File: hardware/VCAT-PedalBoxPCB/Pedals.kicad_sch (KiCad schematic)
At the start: 0 parts

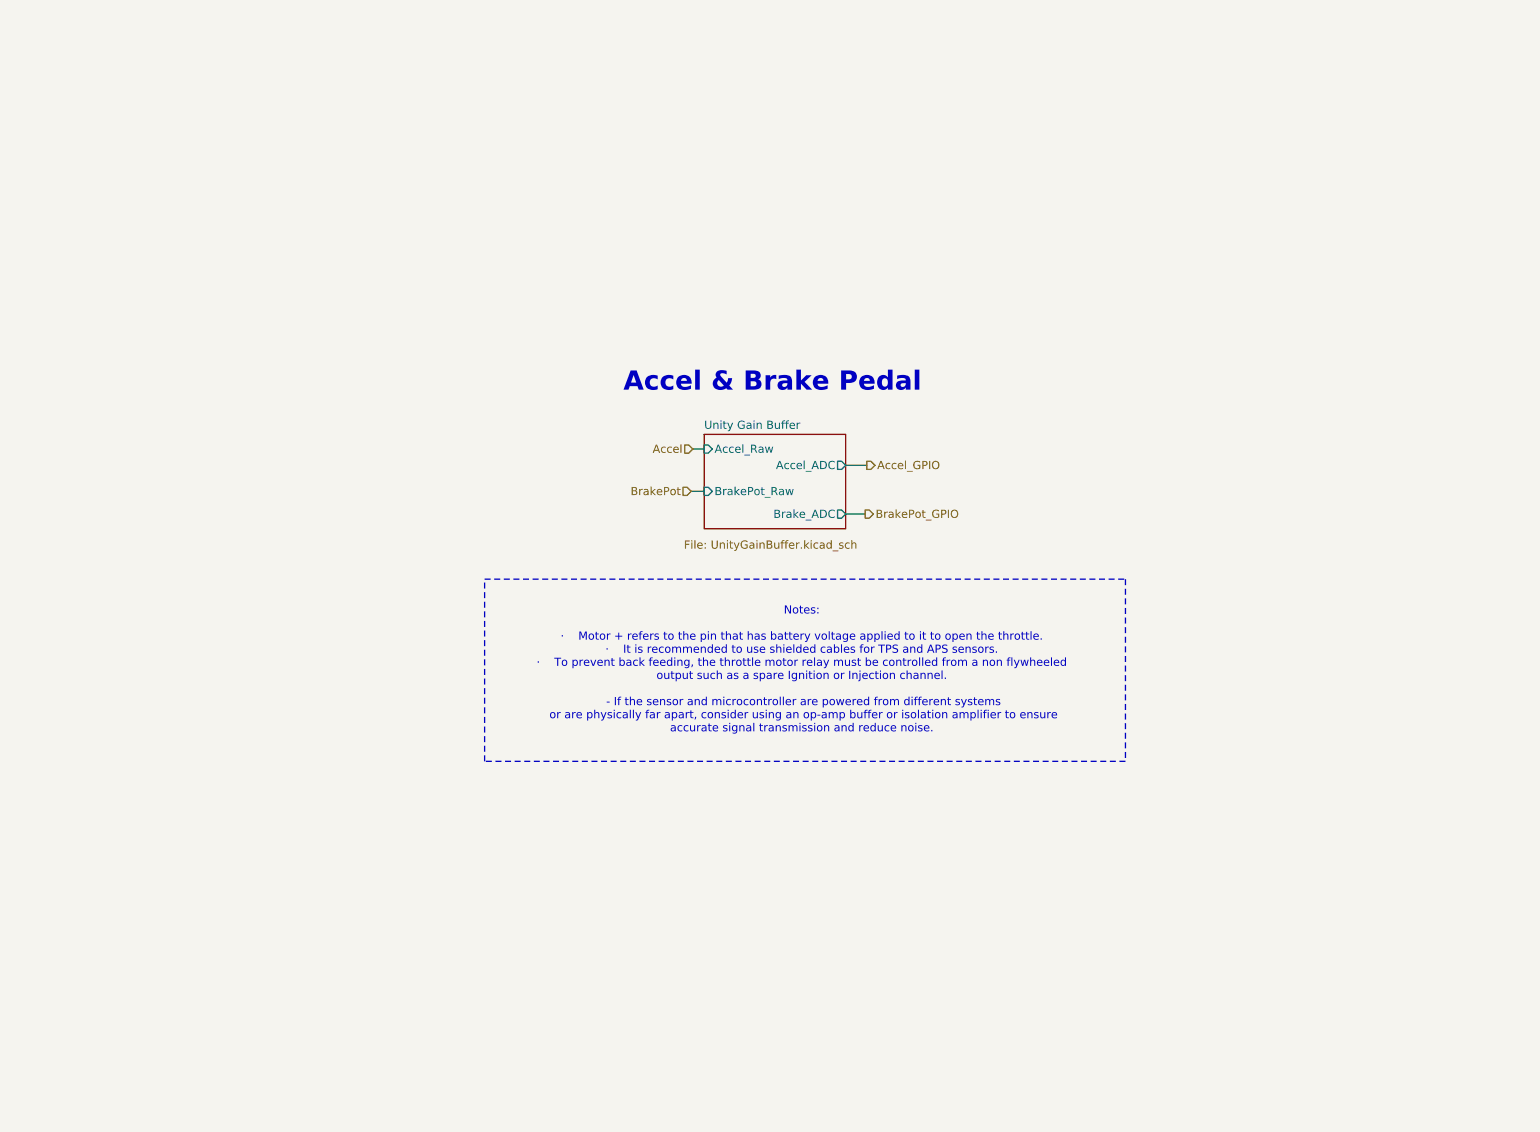
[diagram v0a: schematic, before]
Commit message: Rev B Sch updates
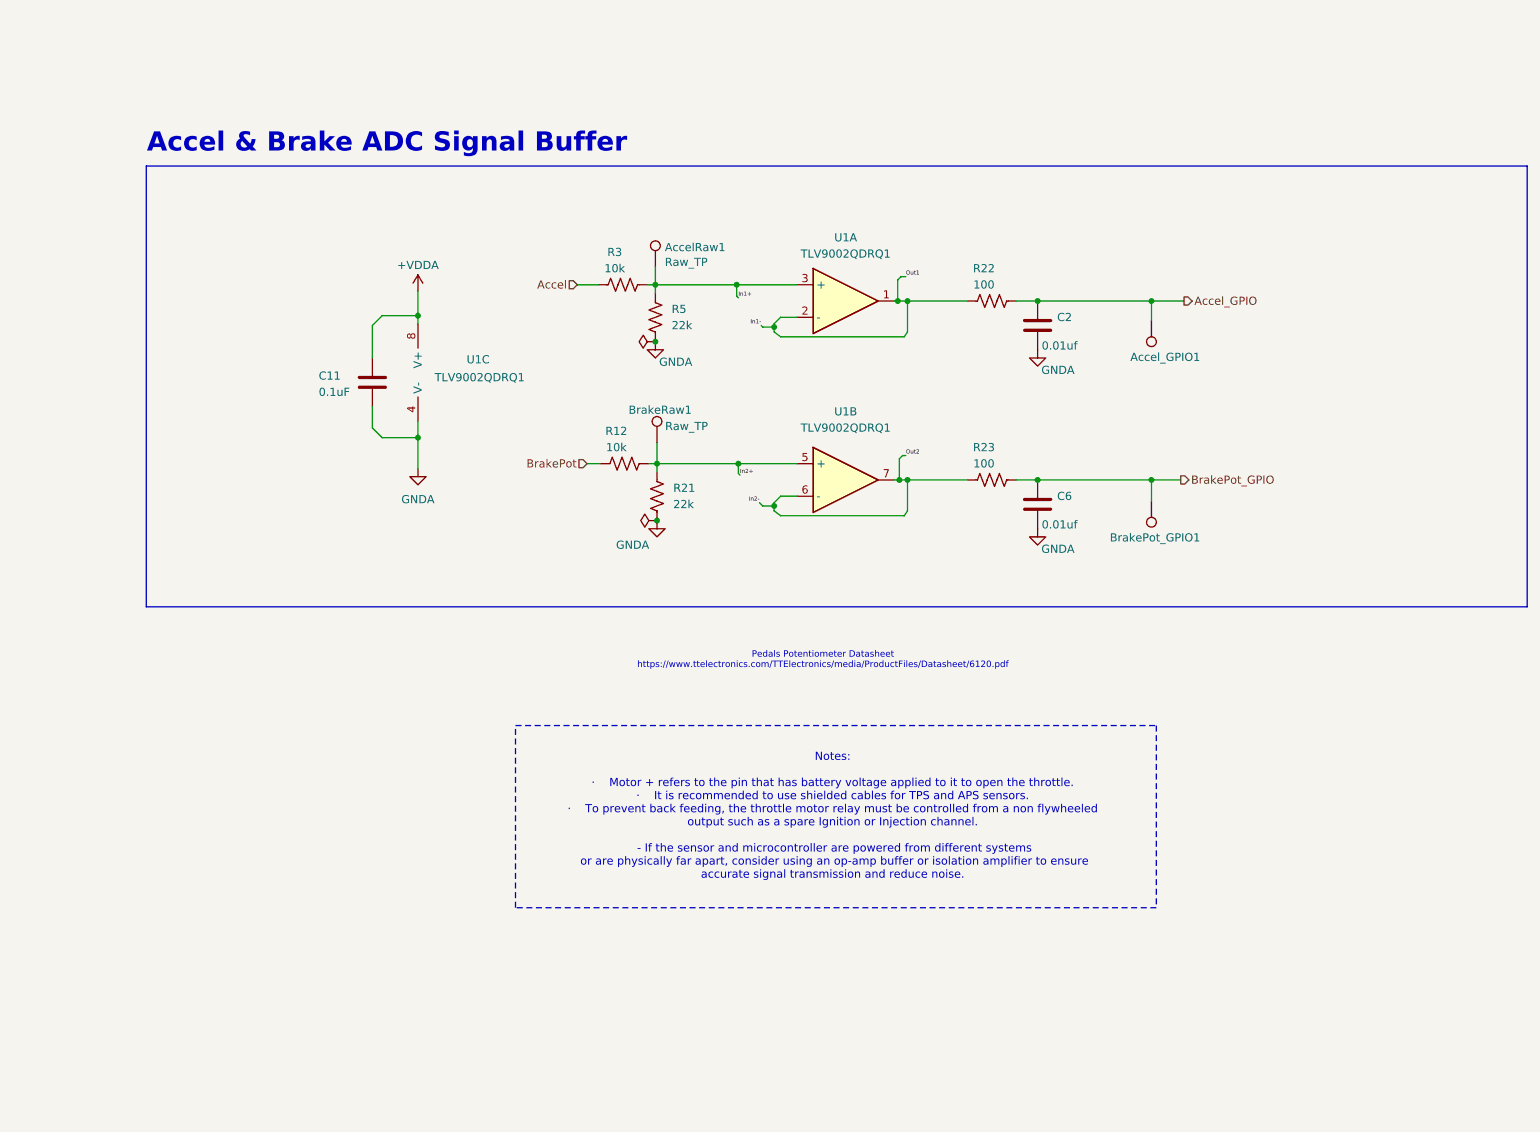
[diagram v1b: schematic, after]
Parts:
- added AccelRaw1, BrakeRaw1: Raw_TP, TestPoint:TestPoint_THTPad_1.5x1.5mm_Drill0.7mm, symbol Connector:TestPoint
- added Accel_GPIO1, BrakePot_GPIO1: Accel, TestPoint:TestPoint_THTPad_1.5x1.5mm_Drill0.7mm, symbol Connector:TestPoint
- added C11: 0.1uF, Capacitor_SMD:C_0603_1608Metric_Pad1.08x0.95mm_HandSolder, symbol Device:C
- added C2, C6: 0.01uf, Capacitor_SMD:C_0603_1608Metric_Pad1.08x0.95mm_HandSolder, symbol Device:C
- added R12, R3: 10k, Resistor_SMD:R_0603_1608Metric_Pad0.98x0.95mm_HandSolder, symbol Device:R_US
- added R21, R5: 22k, Resistor_SMD:R_0603_1608Metric_Pad0.98x0.95mm_HandSolder, symbol Device:R_US
- added R22, R23: 100, Resistor_SMD:R_0603_1608Metric_Pad0.98x0.95mm_HandSolder, symbol Device:R_US
- added U1: TLV9002QDRQ1, TLV9002QDRQ1:SOIC8_D_TEX, symbol Device:Opamp_Dual
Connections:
- net Accel: now also R3.2
- net Accel_GPIO: now also Accel_GPIO1.1, C2.2, R22.1
- net BrakePot: now also R12.2
- net BrakePot_GPIO: now also BrakePot_GPIO1.1, C6.2, R23.1
- new net +VDDA: C11.1, U1.8 (V+)
- new net GNDA: C11.2, C2.1, C6.1, R21.2, R5.2, U1.4 (V-)
- new net In1+: AccelRaw1.1, R3.1, R5.1, U1.3 (+)
- new net In1-: R22.2, U1.1, U1.2 (-)
- new net In2+: BrakeRaw1.1, R12.1, R21.1, U1.5 (+)
- new net In2-: R23.2, U1.6 (-), U1.7
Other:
- removed sheet Unity Gain Buffer
- note added: "Accel & Brake ADC Signal Buffer"
- note added: "Pedals Potentiometer Datasheet https://www.ttelectronics.com/TTElectronics/media/ProductFiles/Datasheet/6120.pdf"
- note removed: "Accel & Brake Pedal"

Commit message: Rev B - Initial Layout
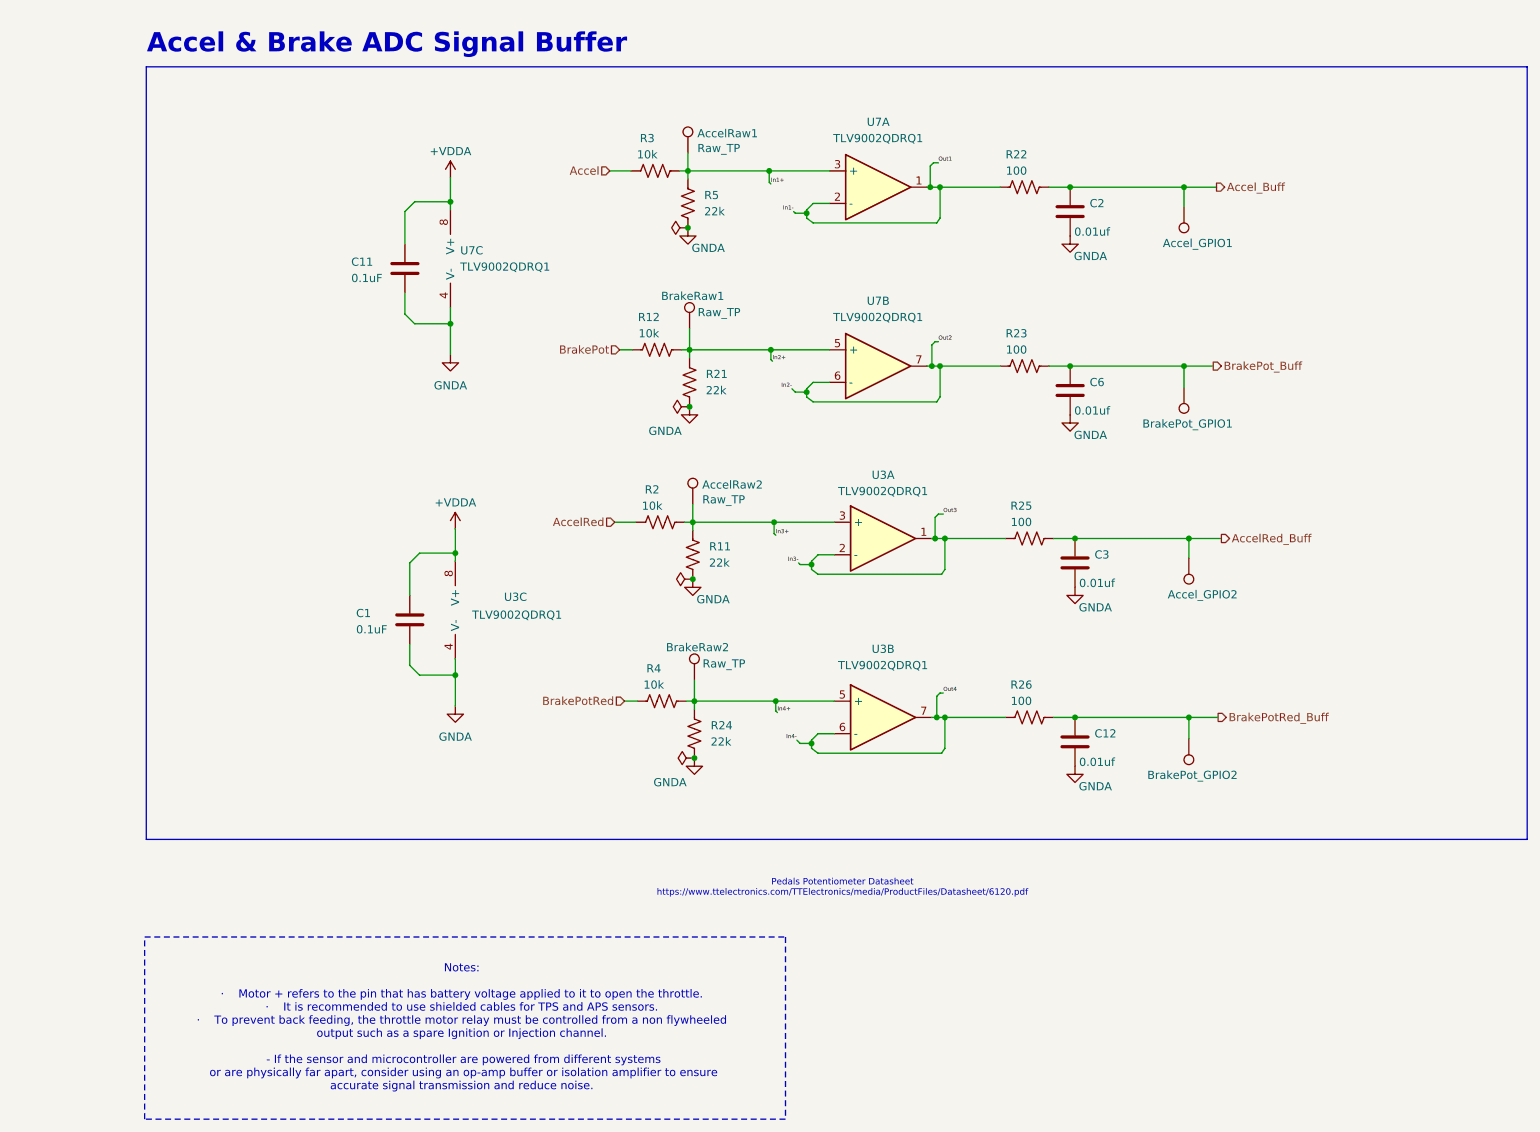
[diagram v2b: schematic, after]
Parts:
- removed U1: TLV9002QDRQ1, TLV9002QDRQ1:SOIC8_D_TEX, symbol Device:Opamp_Dual
- added AccelRaw2, BrakeRaw2: Raw_TP, TestPoint:TestPoint_THTPad_1.5x1.5mm_Drill0.7mm, symbol Connector:TestPoint
- added Accel_GPIO2, BrakePot_GPIO2: Accel, TestPoint:TestPoint_THTPad_1.5x1.5mm_Drill0.7mm, symbol Connector:TestPoint
- added C1: 0.1uF, Capacitor_SMD:C_0603_1608Metric_Pad1.08x0.95mm_HandSolder, symbol Device:C
- added C12, C3: 0.01uf, Capacitor_SMD:C_0603_1608Metric_Pad1.08x0.95mm_HandSolder, symbol Device:C
- added R11, R24: 22k, Resistor_SMD:R_0603_1608Metric_Pad0.98x0.95mm_HandSolder, symbol Device:R_US
- added R2, R4: 10k, Resistor_SMD:R_0603_1608Metric_Pad0.98x0.95mm_HandSolder, symbol Device:R_US
- added R25, R26: 100, Resistor_SMD:R_0603_1608Metric_Pad0.98x0.95mm_HandSolder, symbol Device:R_US
- added U3: TLV9002QDRQ1, TLV9002QDRQ1:SOIC8_D_TEX, symbol Device:Opamp_Dual
- added U7: TLV9002QDRQ1, Package_SO:SOIC-8_3.9x4.9mm_P1.27mm, symbol utsvt_misc:TLV9002QDRQ1
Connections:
- net +VDDA: now also C1.1, U3.8 (V+), U7.8 (V+)
- net GNDA: now also C1.2, C12.1, C3.1, R11.2, R24.2, U3.4 (V-), U7.4 (V-)
- net In1+: now also U7.3 (+)
- net In1-: now also U7.1, U7.2 (-)
- net In2+: now also U7.5 (+)
- net In2-: now also U7.6 (-), U7.7
- net Accel_GPIO renamed Accel_Buff
- net BrakePot_GPIO renamed BrakePot_Buff
- new net AccelRed: R2.2
- new net AccelRed_Buff: Accel_GPIO2.1, C3.2, R25.1
- new net BrakePotRed: R4.2
- new net BrakePotRed_Buff: BrakePot_GPIO2.1, C12.2, R26.1
- new net In3+: AccelRaw2.1, R11.1, R2.1, U3.3 (+)
- new net In3-: R25.2, U3.1, U3.2 (-)
- new net In4+: BrakeRaw2.1, R24.1, R4.1, U3.5 (+)
- new net In4-: R26.2, U3.6 (-), U3.7
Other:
- moved on the sheet: AccelRaw1, Accel_GPIO1, BrakePot_GPIO1, BrakeRaw1, C11, C2, C6, R12, R21, R22, R23, R3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

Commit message: Rev B Sch Review
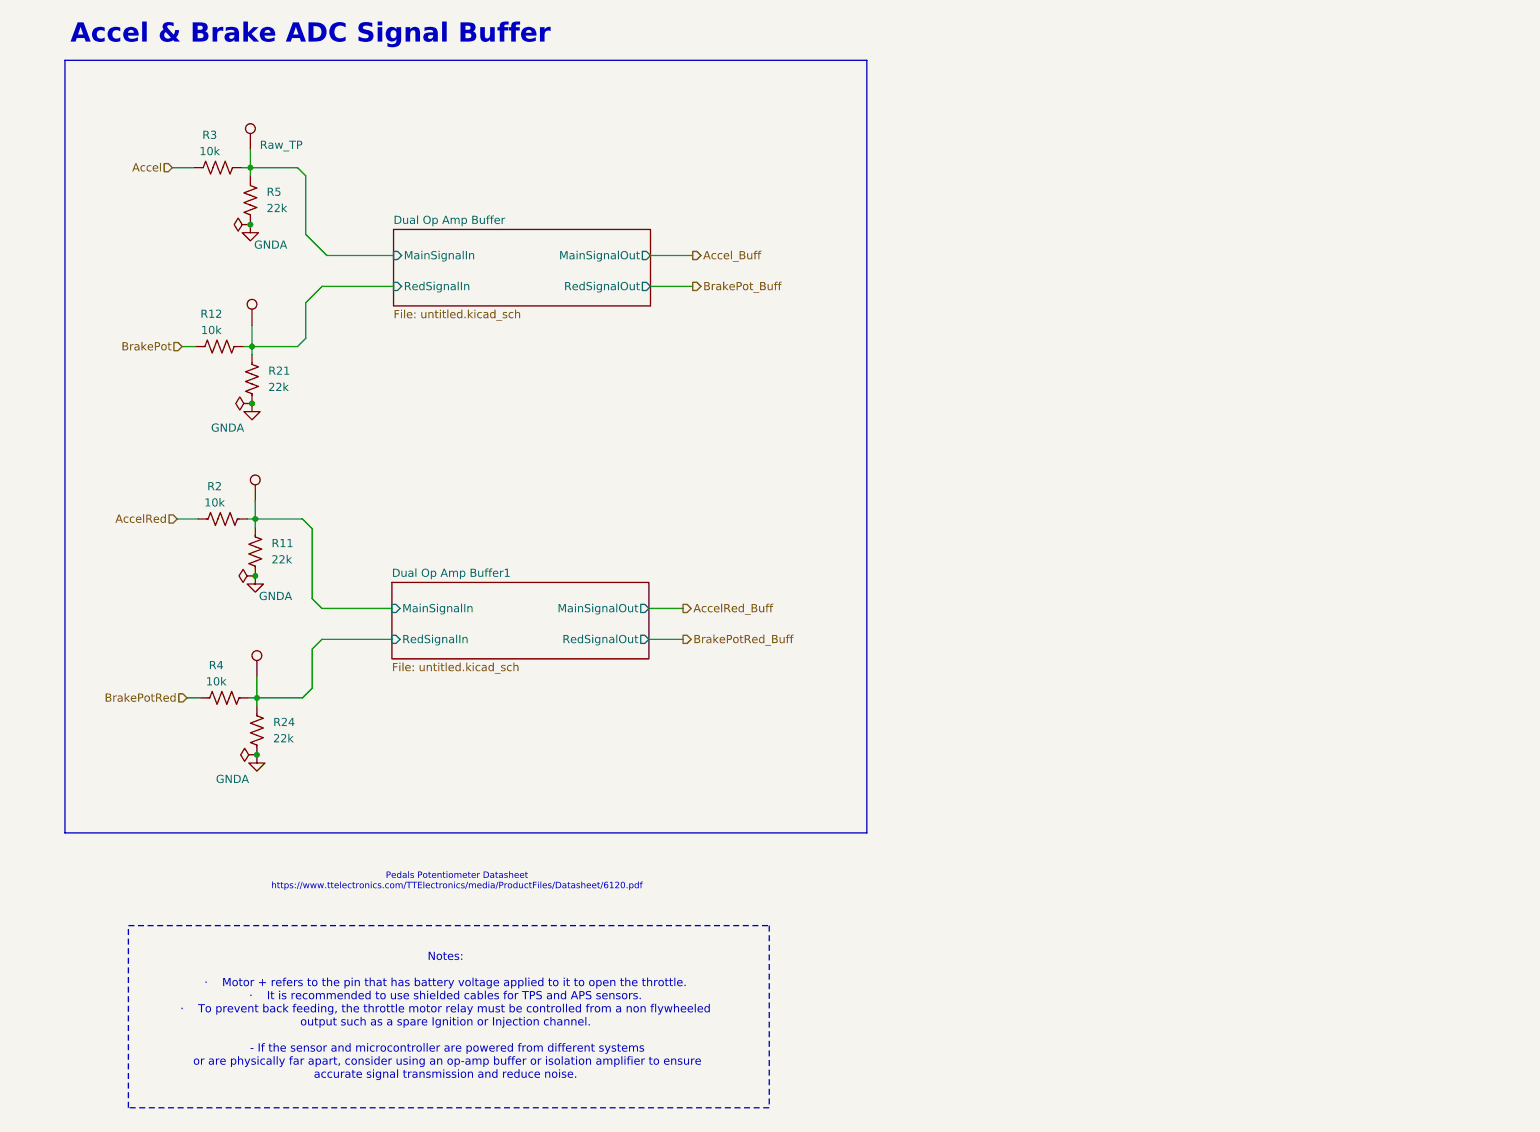
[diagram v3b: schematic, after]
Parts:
- removed Accel_GPIO1, Accel_GPIO2, BrakePot_GPIO1, BrakePot_GPIO2: Accel, TestPoint:TestPoint_THTPad_1.5x1.5mm_Drill0.7mm, symbol Connector:TestPoint
- removed C1, C11: 0.1uF, Capacitor_SMD:C_0603_1608Metric_Pad1.08x0.95mm_HandSolder, symbol Device:C
- removed C12, C2, C3, C6: 0.01uf, Capacitor_SMD:C_0603_1608Metric_Pad1.08x0.95mm_HandSolder, symbol Device:C
- removed R22, R23, R25, R26: 100, Resistor_SMD:R_0603_1608Metric_Pad0.98x0.95mm_HandSolder, symbol Device:R_US
- removed U3: TLV9002QDRQ1, TLV9002QDRQ1:SOIC8_D_TEX, symbol Device:Opamp_Dual
- removed U7: TLV9002QDRQ1, Package_SO:SOIC-8_3.9x4.9mm_P1.27mm, symbol utsvt_misc:TLV9002QDRQ1
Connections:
- net In1+ renamed Dual Op Amp Buffer/MainSignalIn
- net In2+ renamed Dual Op Amp Buffer/RedSignalIn
- net In3+ renamed Dual Op Amp Buffer1/MainSignalIn
- net In4+ renamed Dual Op Amp Buffer1/RedSignalIn
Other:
- added sheet Dual Op Amp Buffer (untitled.kicad_sch)
- added sheet Dual Op Amp Buffer1 (untitled.kicad_sch)
- moved on the sheet: R11, R12, R2, R21, R24, R3, R4, R5
